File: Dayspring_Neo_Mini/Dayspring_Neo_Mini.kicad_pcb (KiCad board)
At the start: 2 copper layers, 170 x 11 mm, 22 parts, among them J1 IN, J2 OUT

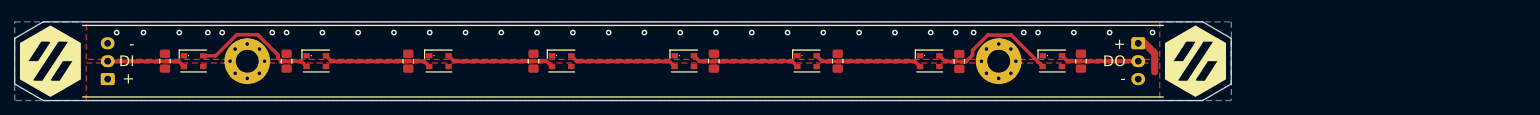
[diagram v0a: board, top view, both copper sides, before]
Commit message: Production Version LED and 3030 Mounts
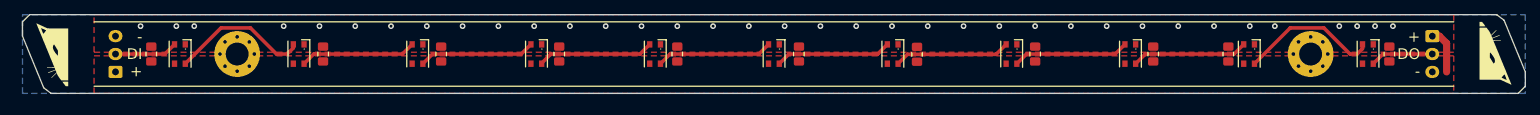
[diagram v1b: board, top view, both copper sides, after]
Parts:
- removed the G*** at (18.0, 33.0)
- removed the G*** at (178.0, 33.0)
- added C10: 0.1uF, Daylight:C_0805_2012Metric_Pad1.18x1.45mm_HandSolder_V3Dspec, F.Cu at (182.6, 32.0)
- added C11: 0.1uF, Daylight:C_0805_2012Metric_Pad1.18x1.45mm_HandSolder_V3Dspec, F.Cu at (205.1, 32.0)
- added C9: 0.1uF, Daylight:C_0805_2012Metric_Pad1.18x1.45mm_HandSolder_V3Dspec, F.Cu at (172.1, 32.0)
- added D10: LED_ALT, Daylight:XL-3528RGBW-WS2812B, F.Cu at (185.5, 32.0)
- added D11: LED_ALT, Daylight:XL-3528RGBW-WS2812B, F.Cu at (202.1, 32.0)
- added D9: LED_ALT, Daylight:XL-3528RGBW-WS2812B, F.Cu at (168.9, 32.0)
- added G***: LOGO, Daylight:RR_Logo_9mm_F-Silk, F.Cu at (218.6, 31.9)
- added G***: LOGO, Daylight:RR_Logo_9mm_F-Silk, F.Cu at (19.6, 32.1)
- moved H2 43.6 mm to (194.1, 32.0)
- moved J2 41.1 mm to (211.1, 29.5)
- moved C8 6.49 mm to (155.6, 32.0)
- moved C7 5.99 mm to (139.1, 32.0)
- moved D8 5.80 mm to (152.3, 32.0), turned to 90 degrees
- moved C6 5.50 mm to (122.6, 32.0)
- moved D7 5.26 mm to (135.7, 32.0), turned to 90 degrees
- moved C5 5.21 mm to (105.6, 32.0)
- moved C2 5.19 mm to (56.1, 32.0)
- moved D6 4.73 mm to (119.1, 32.0), turned to 90 degrees
- moved C3 4.70 mm to (72.6, 32.0)
- moved D5 4.20 mm to (102.5, 32.0), turned to 90 degrees
- moved C4 3.73 mm to (89.1, 32.0)
- moved D4 3.68 mm to (85.9, 32.0), turned to 90 degrees
- moved D3 3.16 mm to (69.3, 32.0), turned to 90 degrees
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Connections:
- D8 pad 4: Dend -> Net-(D8-Pad4)
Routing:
- net Net-(D10-Pad4): track 0.00 -> 19.6 mm
- net Net-(D10-Pad2): track 0.00 -> 16.2 mm
- net Net-(D8-Pad4): track 0.00 -> 16.2 mm
- net Net-(D7-Pad4): track 18.5 -> 16.2 mm
- net Dend: track 11.0 -> 8.81 mm
- net Dstart: track 11.0 -> 8.81 mm
- net Net-(D1-Pad4): track 17.8 -> 19.5 mm
- net Net-(D4-Pad4): track 15.1 -> 16.3 mm
- net Net-(D5-Pad4): track 15.1 -> 16.2 mm
- net Net-(D6-Pad4): track 15.1 -> 16.2 mm
- net Net-(D2-Pad4): track 15.1 -> 16.2 mm
- net Net-(D3-Pad4): track 15.1 -> 16.2 mm
- net +5V: track 5.48 -> 6.41 mm
- net GND: vias 32 -> 36
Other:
- board size 170 x 11 mm -> 210 x 11 mm
